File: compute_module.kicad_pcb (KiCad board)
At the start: 4 copper layers, 93.2 x 62.4 mm, 66 parts, among them J1 2001-1-2-21-00-BK, J2 JC-128, P1 POWER, P2 HOST, P3 CAM1, P4 CONN_02X20, Q1 2N7002P.215, Q2 DMP3056L-7, Q3 2N7002P.215, U1 REG1117-3.3, U3 REG1117A-1.8

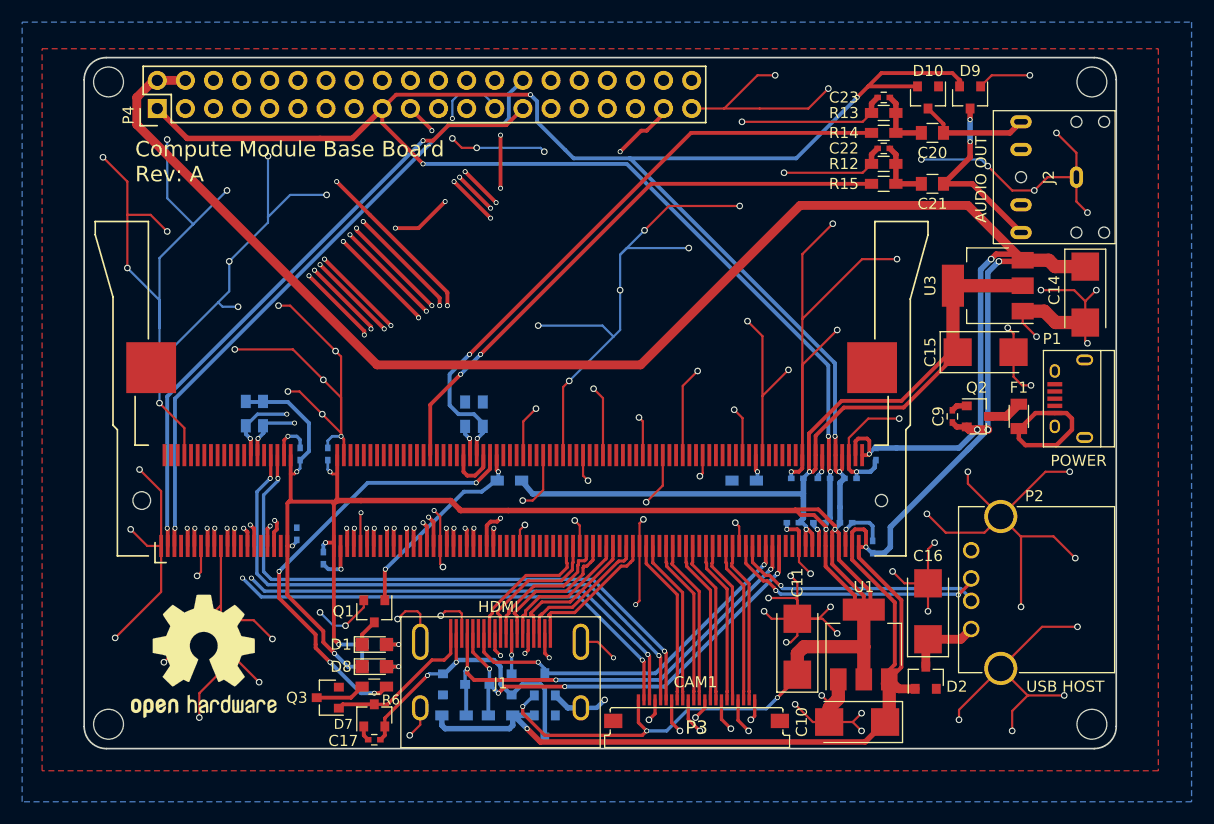
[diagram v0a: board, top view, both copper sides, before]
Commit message: migrate pcb
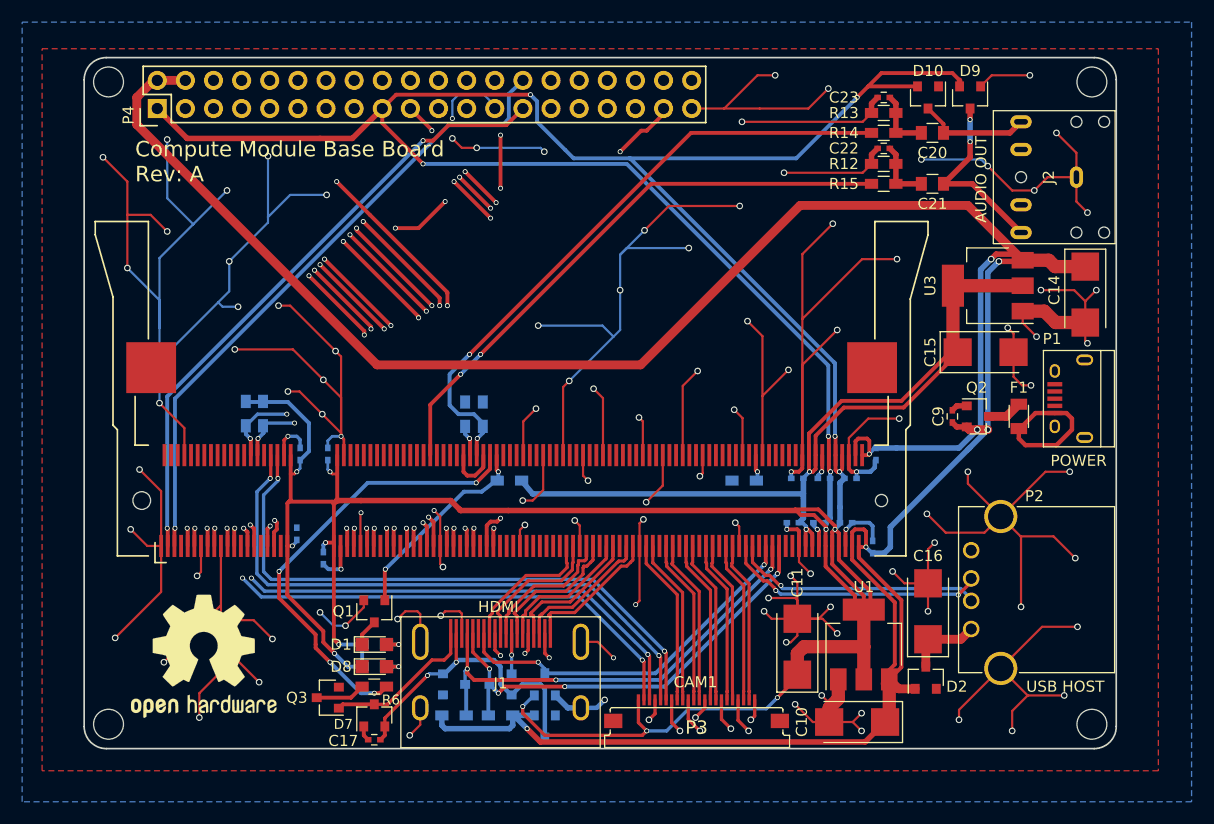
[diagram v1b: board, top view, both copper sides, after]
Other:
- net class Default removed
